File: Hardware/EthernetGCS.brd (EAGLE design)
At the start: 73.7 x 42.2 mm, 67 parts, among them IC3 24AA00OT, IC4 PIC24FJ64GA002_QFN, J2 HR911105A, Q2 25Mhz, U1 MIC5219-3.3V, U3 MIC5219-3.3V, U4 ENC28J60-QFN, U5 MIC5219-3.3V, U7 FT232RL-BASICSSOP, X2 USB-A-H

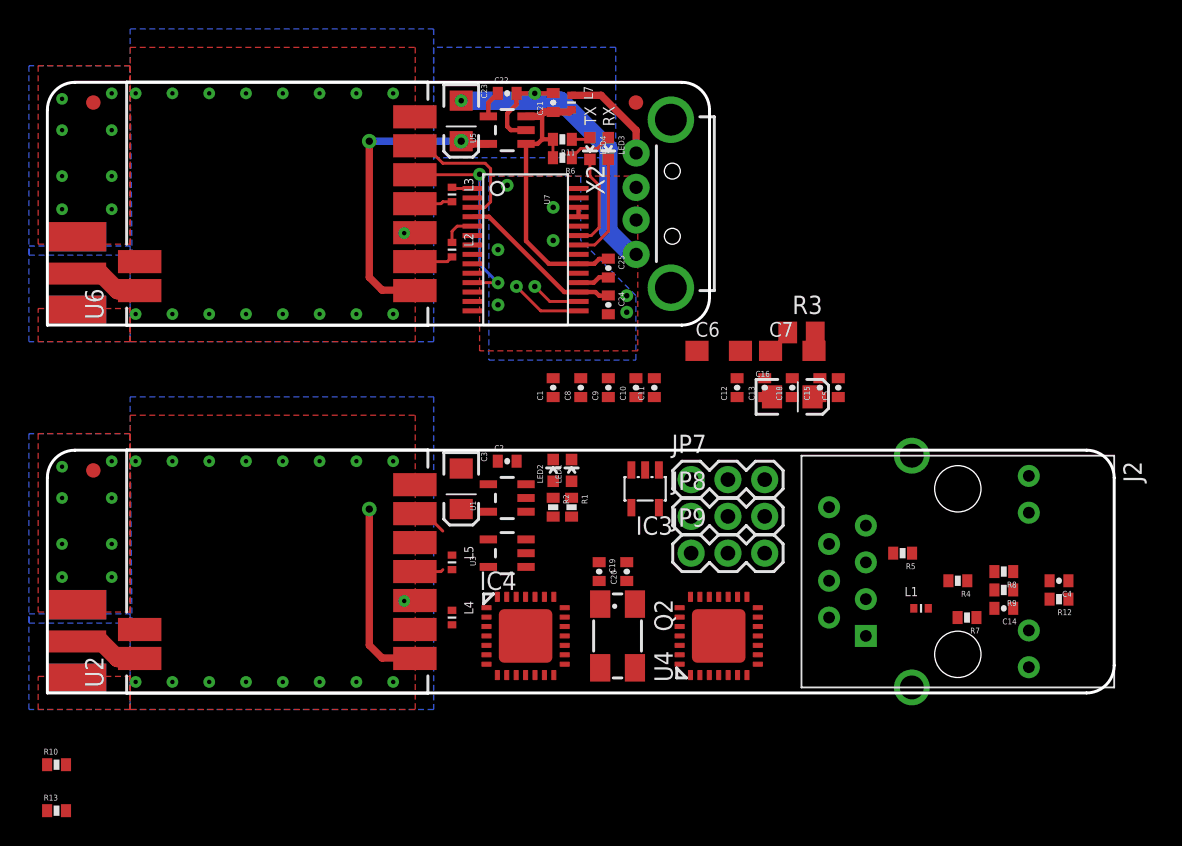
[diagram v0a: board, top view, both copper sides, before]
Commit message: Just moving some parts to easy  layout process.
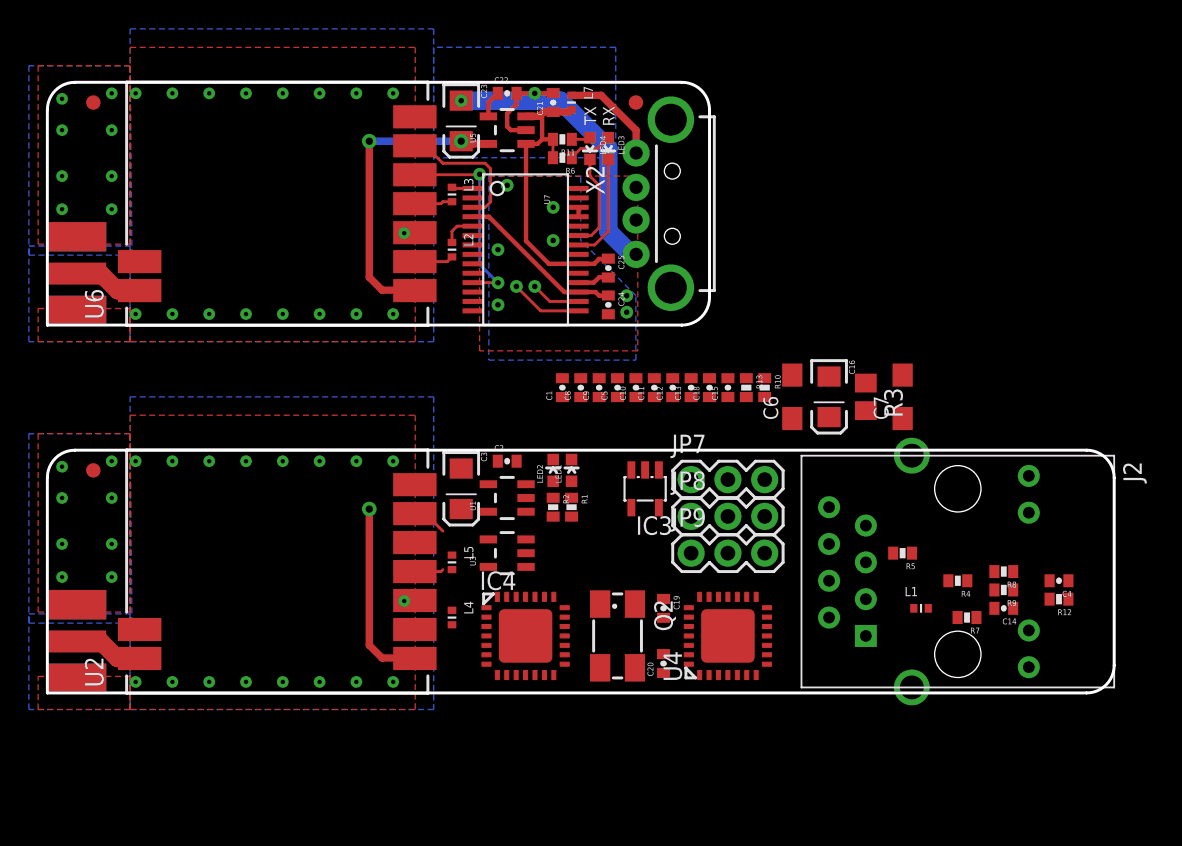
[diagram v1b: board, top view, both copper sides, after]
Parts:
- moved R13 55.9 mm to (48.3, 21.6), turned to 270 degrees
- moved R10 55.4 mm to (49.5, 21.6), turned to 270 degrees
- moved C5 15.2 mm to (39.4, 21.6)
- moved C7 8.25 mm to (59.1, 21.0), turned to 90 degrees
- moved C20 6.84 mm to (42.5, 2.54)
- moved C15 6.35 mm to (47.0, 21.6)
- moved R3 6.29 mm to (56.5, 21.0), turned to 270 degrees
- moved C6 5.99 mm to (51.4, 21.0), turned to 90 degrees
- moved C18 5.72 mm to (45.7, 21.6)
- moved C19 5.12 mm to (42.5, 6.35)
- moved C13 5.08 mm to (44.5, 21.6)
- moved C12 4.45 mm to (43.2, 21.6)
- moved C16 2.54 mm to (54.0, 21.0), turned to 270 degrees
- moved C1 0.64 mm to (35.6, 21.6)
- moved U4 0.64 mm to (47.0, 4.45)
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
